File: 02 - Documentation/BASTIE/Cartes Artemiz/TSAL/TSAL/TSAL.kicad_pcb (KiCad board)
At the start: 2 copper layers, 58 x 58 mm, 125 parts, among them J1 2P Droit 2-11-2022, J2 2P Droit 2-11-2022, J3 2P Droit 2-11-2022, J4 3P Droit 22-11-2032, J5 2P Droit 2-11-2022, J6 2P Droit 2-11-2022, J7 4P Droit 22-11-2042, J8 3P Droit 22-11-2032, J9 2P Droit 2-11-2022, Q1 NMOS SQ2348ES-T1_GE3, Q2 NMOS SQ2348ES-T1_GE3, Q3 PMOS SI2343CDS-T1-GE3, Q4 PMOS SI2343CDS-T1-GE3, U1 Opamp_Quad, U2 Opamp

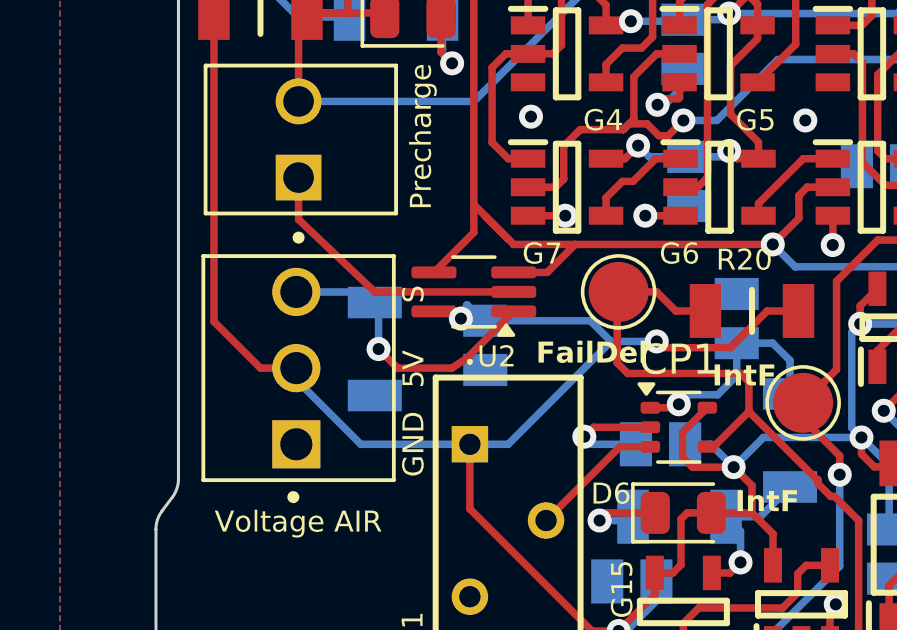
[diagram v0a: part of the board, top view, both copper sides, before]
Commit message: Aop fixes
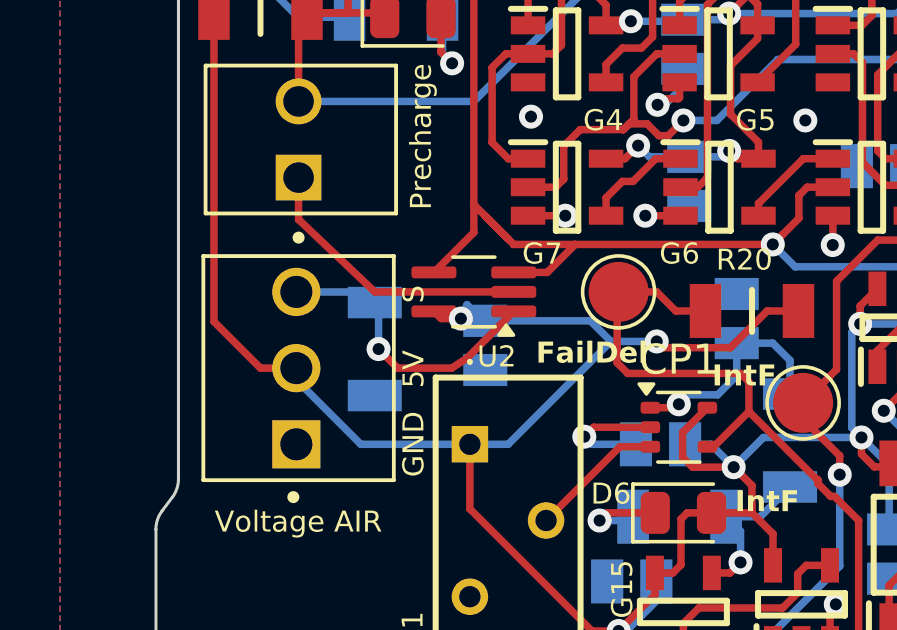
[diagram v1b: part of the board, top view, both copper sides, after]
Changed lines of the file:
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@@
-	)
-	(segment
-		(start 108.6762 67.325)
-		(end 108.9152 67.564)
-		(width 0.25)
-		(layer "F.Cu")
-		(net 1)
 	)
 	(segment
@@
 	)
 	(segment
+		(start 108.256 67.564)
+		(end 108.017 67.325)
+		(width 0.25)
+		(layer "F.Cu")
+		(net 1)
+	)
+	(segment
 		(start 144.26232 53.83832)
 		(end 144.26232 61.98568)
@@
 	)
 	(segment
+		(start 108.9152 67.564)
+		(end 108.256 67.564)
+		(width 0.25)
+		(layer "F.Cu")
+		(net 1)
+	)
+	(segment
 		(start 118.805 53.345)
 		(end 117.8645 53.345)
@@
 		(width 0.25)
 		(layer "F.Cu")
-		(net 1)
-	)
-	(segment
-		(start 108.017 67.325)
-		(end 108.6762 67.325)
-		(width 0.25)
-		(layer "F.Cu")
